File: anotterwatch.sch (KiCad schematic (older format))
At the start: 51 parts, among them J3 Micro_SD_Card, Q1 AO3400, Q2 AO3400, Q3 npn, Q4 npn, Q7 AO3400, U1 TP4056, U12 BMI270, U2 ESP32, U3 CH340C, U4 ST7789V

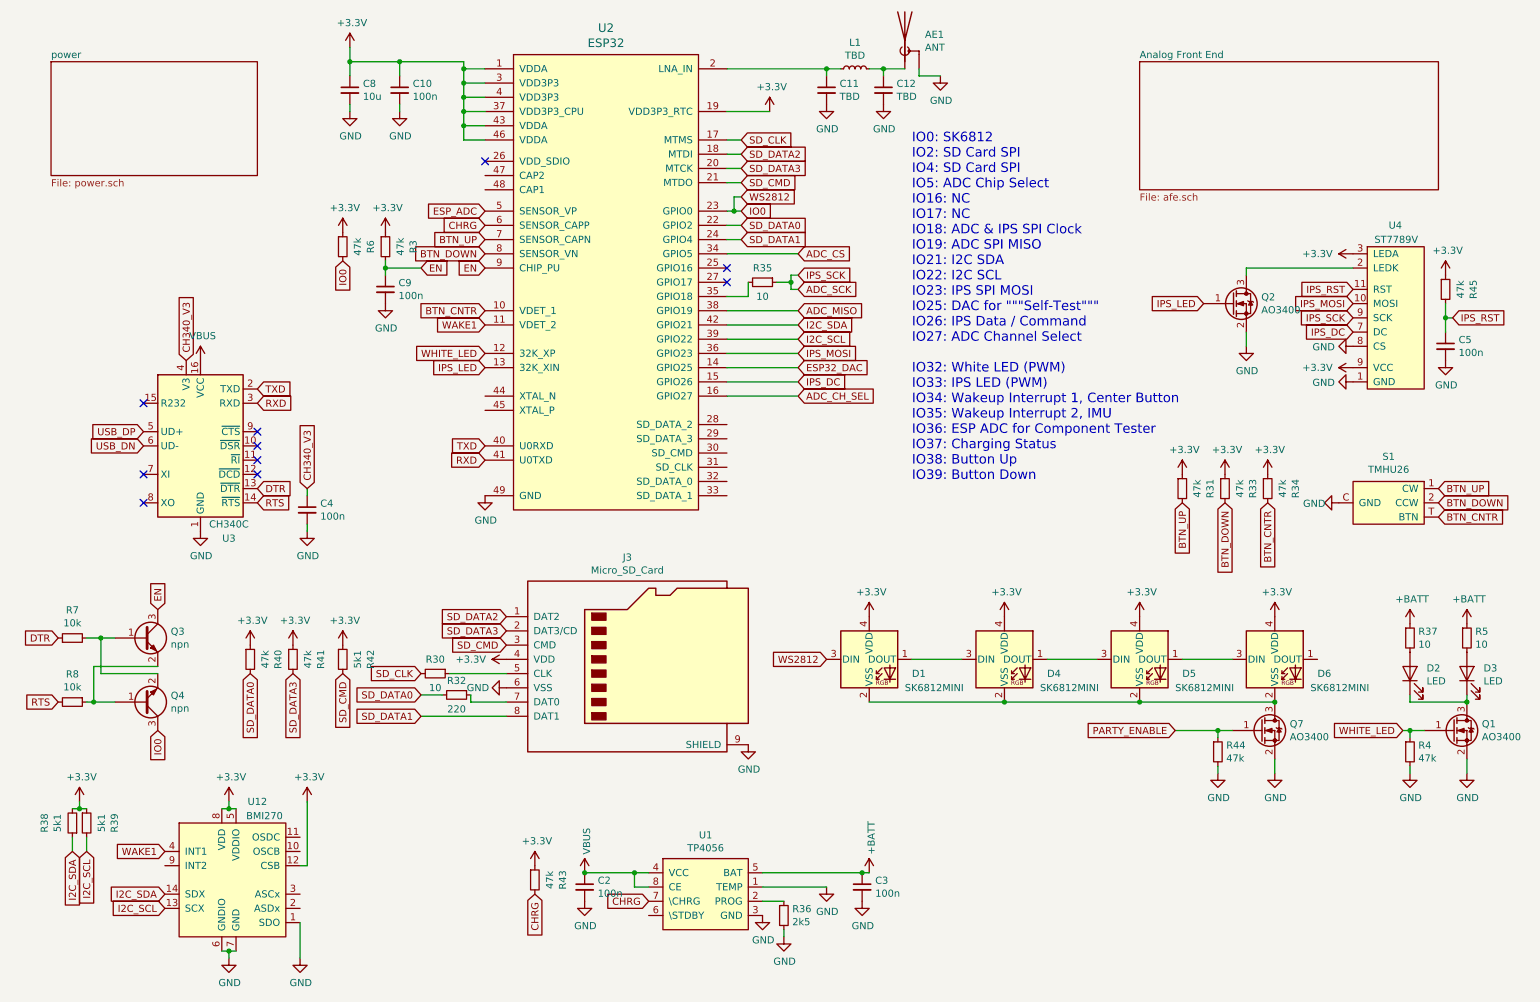
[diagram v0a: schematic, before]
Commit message: Schematic cleanup
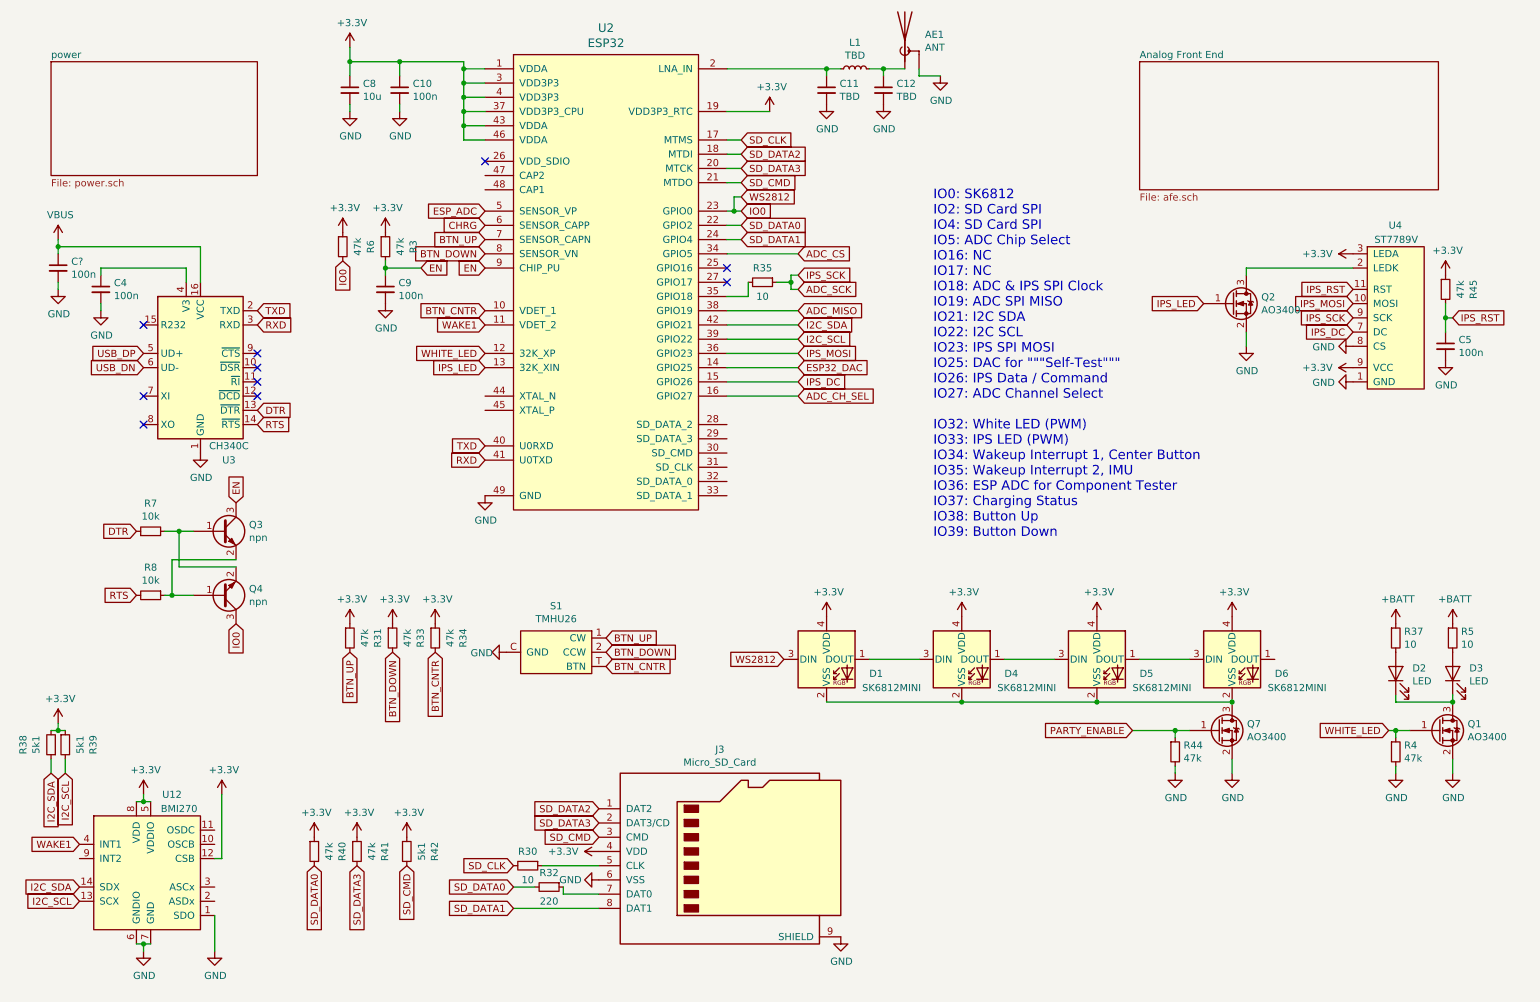
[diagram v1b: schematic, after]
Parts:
- removed C2, C3: 100n, Capacitor_SMD:C_0603_1608Metric, symbol Device:C_Small
- removed R36: 2k5, Resistor_SMD:R_0603_1608Metric, symbol Device:R_Small
- removed R43: 47k, Resistor_SMD:R_0603_1608Metric, symbol Device:R_Small
- removed U1: TP4056, symbol badgelib:TP4056
- added C?: 100n, Capacitor_SMD:C_0603_1608Metric, symbol Device:C_Small
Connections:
- net GND: now also C?.2
- net VBUS: now also C?.1
- net CH340_V3: no longer names the net of C4.1, U3.4 (V3)
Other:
- moved on the sheet: C4, D1, D2, D3, D4, D5, D6, J3, Q1, Q3, Q4, Q7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
